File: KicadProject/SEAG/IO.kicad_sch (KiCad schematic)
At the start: 12 parts, among them J10 Screw_Terminal_01x02, J3 Screw_Terminal_01x02, J4 Screw_Terminal_01x02, J5 Screw_Terminal_01x02, J6 Screw_Terminal_01x02, J7 Screw_Terminal_01x02, J8 Screw_Terminal_01x02, J9 Screw_Terminal_01x02

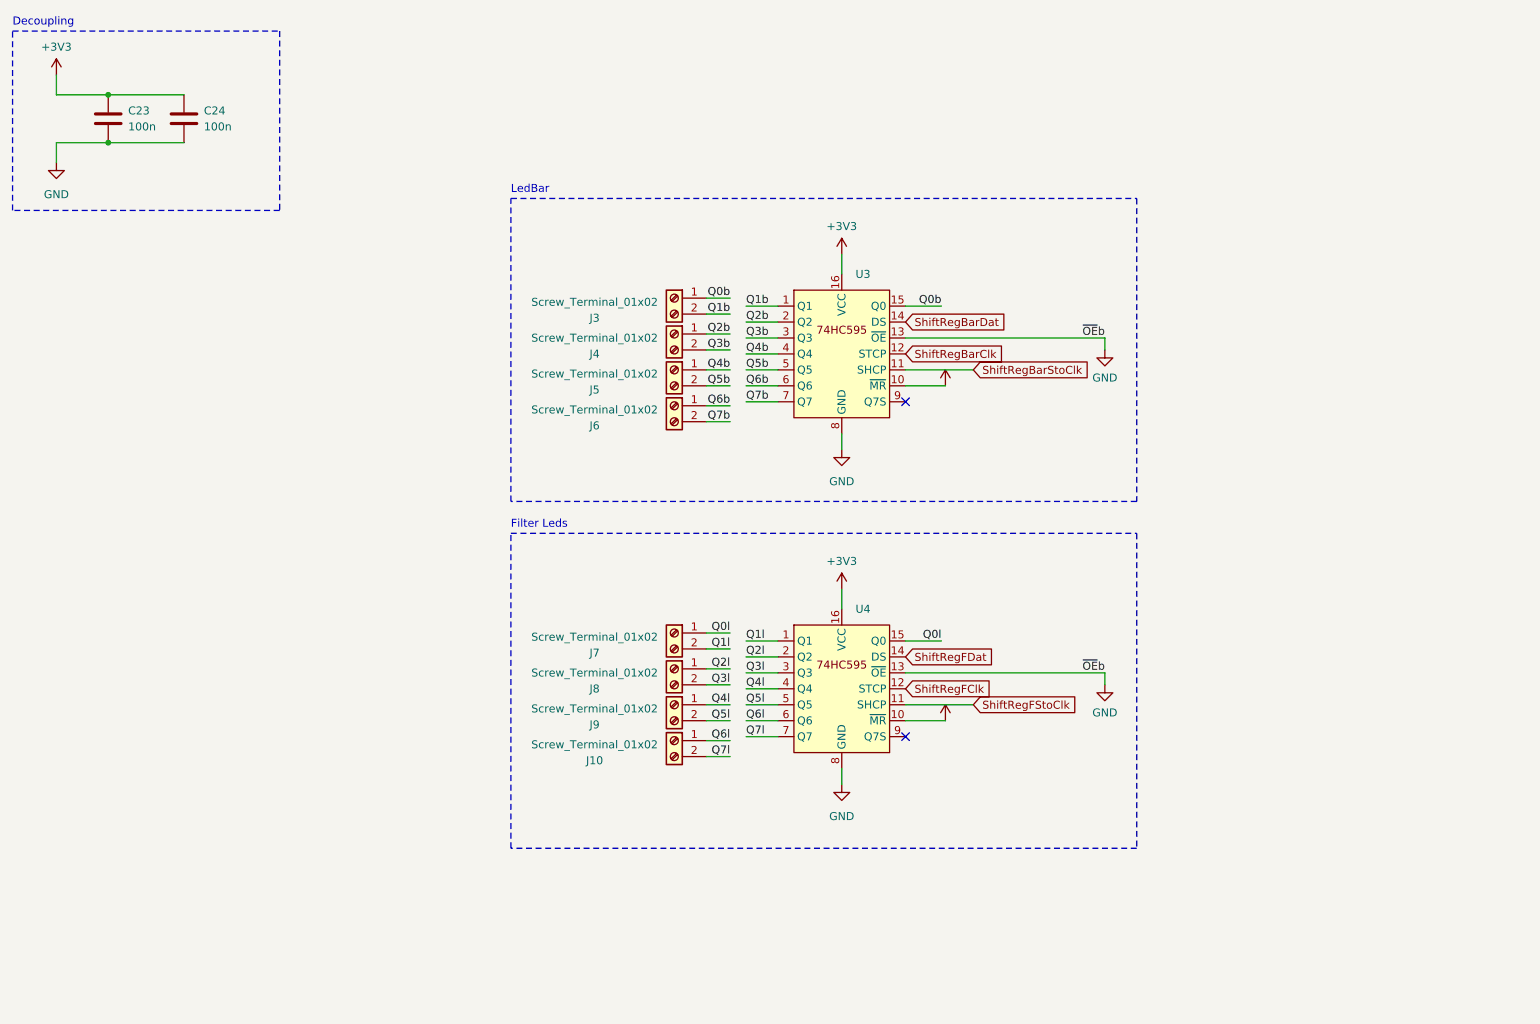
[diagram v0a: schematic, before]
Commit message: PCB rev 2
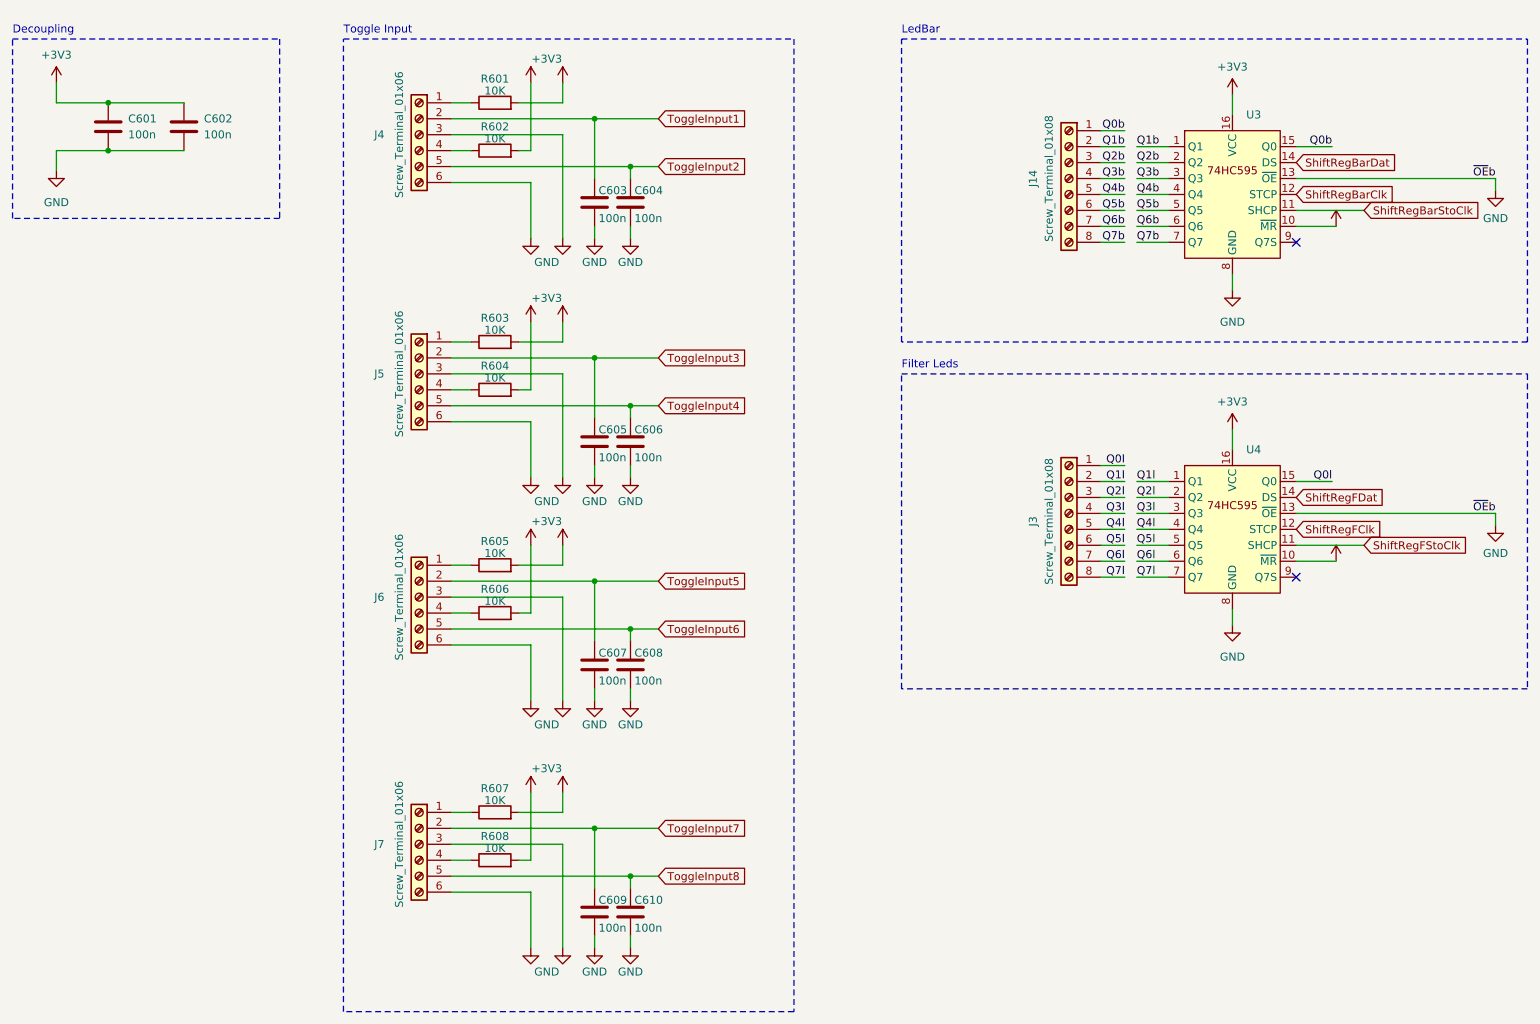
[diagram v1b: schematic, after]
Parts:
- removed J10, J3, J4, J5, J6, J7, J8, J9: Screw_Terminal_01x02, TerminalBlock_Phoenix:TerminalBlock_Phoenix_MKDS-1,5-2_1x02_P5.00mm_Horizontal, symbol Connector:Screw_Terminal_01x02
- added C603, C604, C605, C606, C607, C608, C609, C610: 100n, Capacitor_SMD:C_0805_2012Metric, symbol Device:C
- added J14, J3: Screw_Terminal_01x08, SamacSys_Parts:1725711, symbol Connector:Screw_Terminal_01x08
- added J4, J5, J6, J7: Screw_Terminal_01x06, SamacSys_Parts:1725698, symbol Connector:Screw_Terminal_01x06
- added R601, R602, R603, R604, R605, R606, R607, R608: 10K, Resistor_SMD:R_0805_2012Metric, symbol Device:R
- renumbered C23 to C601, C24 to C602
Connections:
- net +3V3: now also R601.2, R602.2, R603.2, R604.2, R605.2, R606.2, R607.2, R608.2
- net GND: now also C603.2, C604.2, C605.2, C606.2, C607.2, C608.2, C609.2, C610.2, J4.3 (Pin_3), J4.6 (Pin_6), J5.3 (Pin_3), J5.6 (Pin_6), J6.3 (Pin_3), J6.6 (Pin_6), J7.3 (Pin_3), J7.6 (Pin_6)
- net Q0b: now also J14.1 (Pin_1)
- net Q0l: now also J3.1 (Pin_1)
- net Q1b: now also J14.2 (Pin_2)
- net Q1l: now also J3.2 (Pin_2)
- net Q2b: now also J14.3 (Pin_3)
- net Q2l: now also J3.3 (Pin_3)
- net Q3b: now also J14.4 (Pin_4)
- net Q3l: now also J3.4 (Pin_4)
- net Q4b: now also J14.5 (Pin_5)
- net Q4l: now also J3.5 (Pin_5)
- net Q5b: now also J14.6 (Pin_6)
- net Q5l: now also J3.6 (Pin_6)
- net Q6b: now also J14.7 (Pin_7)
- net Q6l: now also J3.7 (Pin_7)
- net Q7b: now also J14.8 (Pin_8)
- net Q7l: now also J3.8 (Pin_8)
- new net: J7.4 (Pin_4), R608.1
- new net: J7.1 (Pin_1), R607.1
- new net: J4.1 (Pin_1), R601.1
- new net: J6.4 (Pin_4), R606.1
- new net: J5.1 (Pin_1), R603.1
- new net: J5.4 (Pin_4), R604.1
- new net: J4.4 (Pin_4), R602.1
- new net: J6.1 (Pin_1), R605.1
- new net ToggleInput1: C603.1, J4.2 (Pin_2)
- new net ToggleInput2: C604.1, J4.5 (Pin_5)
- new net ToggleInput3: C605.1, J5.2 (Pin_2)
- new net ToggleInput4: C606.1, J5.5 (Pin_5)
- new net ToggleInput5: C607.1, J6.2 (Pin_2)
- new net ToggleInput6: C608.1, J6.5 (Pin_5)
- new net ToggleInput7: C609.1, J7.2 (Pin_2)
- new net ToggleInput8: C610.1, J7.5 (Pin_5)
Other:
- note added: "Toggle Input"
- moved on the sheet: C601, C602, U3, U4
